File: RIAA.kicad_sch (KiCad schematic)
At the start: 65 parts, among them K1 G6K-2, P10 From Keyboard, P8 From main PCB, P9 From Wire, Q1 Q_NPN_BCE, U5 OPA2134, U6 OPA2134, U7 LM317_TO-220

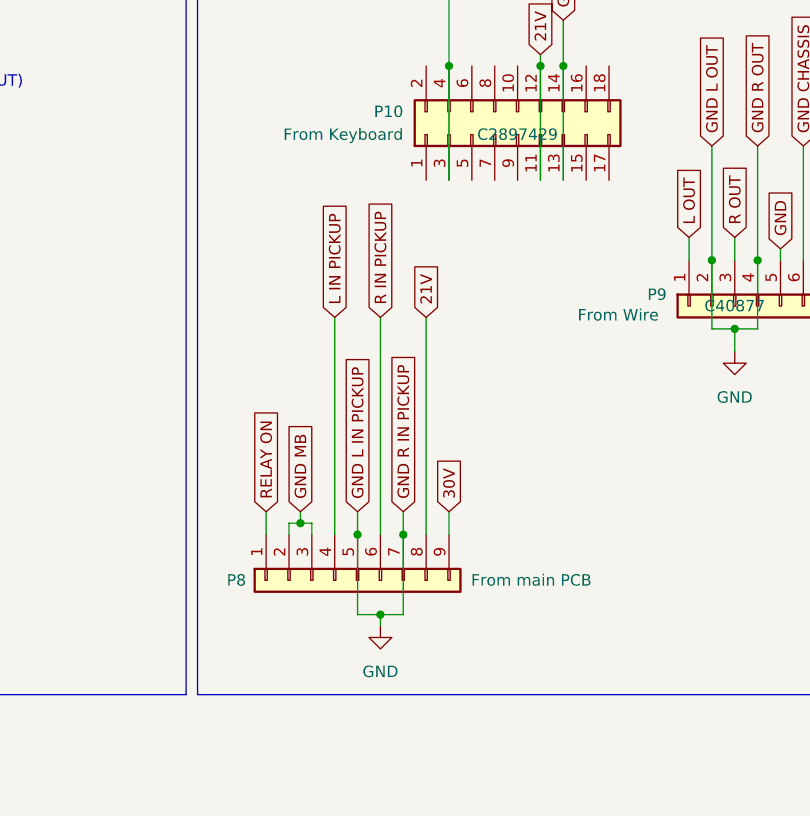
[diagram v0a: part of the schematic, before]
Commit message: WIP: Finishing up SMD version.
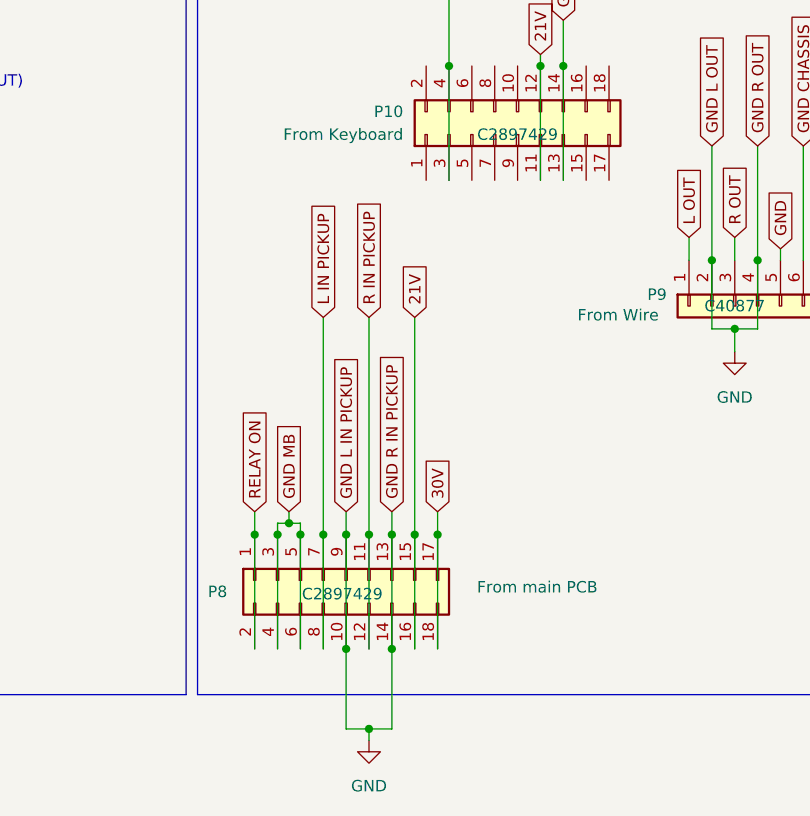
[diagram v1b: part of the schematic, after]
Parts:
- removed P8: From main PCB, Connector_PinSocket_2.54mm:PinSocket_1x09_P2.54mm_Horizontal, symbol Connector_Generic:Conn_01x09
- added P8: From main PCB, Connector_PinSocket_2.54mm:PinSocket_2x09_P2.54mm_Horizontal, symbol Connector_Generic:Conn_02x09_Odd_Even
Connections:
- net 21V: now also P8.15 (Pin_15), P8.16 (Pin_16)
- net 30V: now also P8.17 (Pin_17), P8.18 (Pin_18)
- net GND: now also P8.10 (Pin_10), P8.13 (Pin_13), P8.14 (Pin_14), P8.3 (Pin_3), P8.4 (Pin_4), P8.5 (Pin_5), P8.6 (Pin_6), P8.9 (Pin_9)
- net L IN PICKUP: now also P8.7 (Pin_7), P8.8 (Pin_8)
- net R IN PICKUP: now also P8.11 (Pin_11), P8.12 (Pin_12)
- net RELAY ON: now also P8.1 (Pin_1), P8.2 (Pin_2)
